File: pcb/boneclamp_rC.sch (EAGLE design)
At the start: 133 parts, among them U1 OPA365AIDBVR, U10 AD5686, U11 LM2663, U12 MAX1735, U13 TLV70245, U14 REF5040MDREP, U15 AD8032ARZ-REEL7, U16 24C, U2 OPA365AIDBVR, U3 OPA365AIDBVR, U4 OPA365AIDBVR, U5 ADS8331IBPW, U6 OPA365AIDBVR, U7 OPA365, U8 OPA365AIDBVR, U9 OPA365AIDBVR

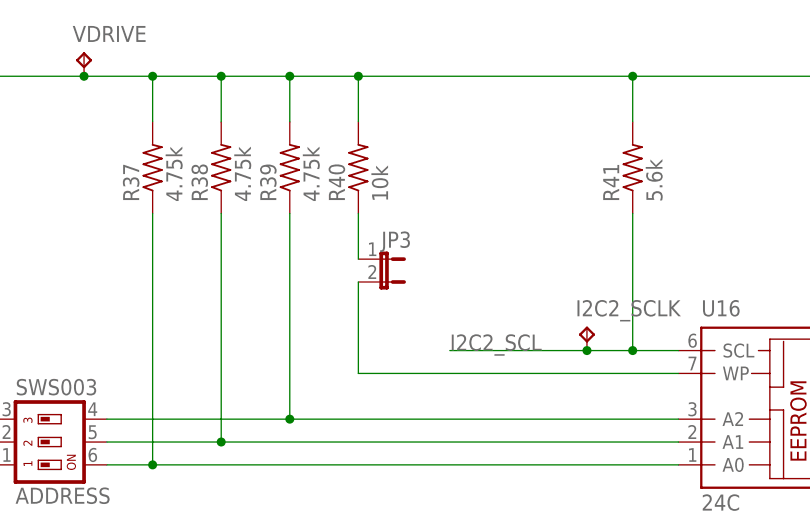
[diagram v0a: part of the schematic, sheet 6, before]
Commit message: Finished basic DAC buffer layout.
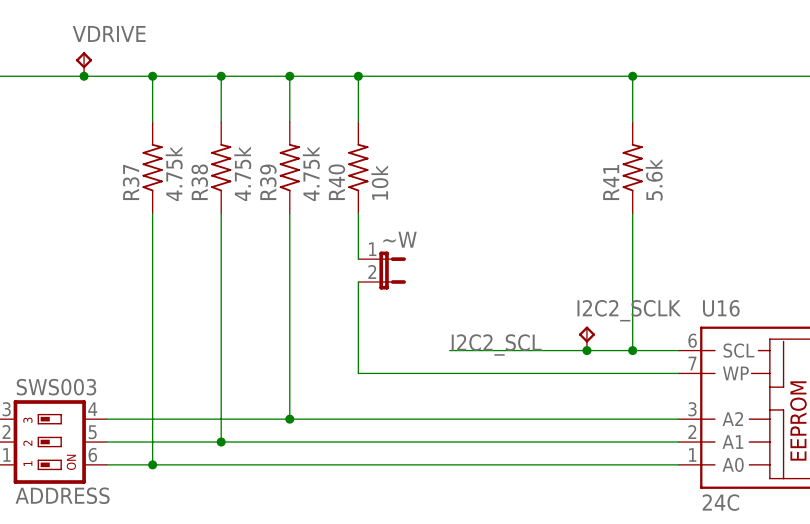
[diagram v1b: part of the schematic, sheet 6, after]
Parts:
- renumbered JP3 to ~W
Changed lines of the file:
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@@
 <part name="SUPPLY10" library="supply2" deviceset="AGND" device=""/>
 <part name="SUPPLY2" library="supply2" deviceset="AGND" device=""/>
-<part name="JP3" library="jumper" deviceset="JP1E" device=""/>
+<part name="~W" library="jumper" deviceset="JP1E" device=""/>
 <part name="ADDRESS" library="smd-special" deviceset="SWS003" device=""/>
 <part name="I2C2_SDA" library="testpad" deviceset="TP" device="B1,27"/>
@@
 <instance part="I2C2_SCLK" gate="G$1" x="-25.4" y="33.02"/>
 <instance part="VDRIVE" gate="G$1" x="-81.28" y="63.5"/>
-<instance part="JP3" gate="A" x="-48.26" y="40.64" rot="R270"/>
+<instance part="~W" gate="A" x="-48.26" y="40.64" rot="R270"/>
 <instance part="ADDRESS" gate="G$1" x="-86.36" y="20.32" rot="MR90"/>
 <instance part="I2C2_SDA" gate="G$1" x="15.24" y="25.4"/>
@@
 <segment>
 <pinref part="R40" gate="G$1" pin="1"/>
-<pinref part="JP3" gate="A" pin="1"/>
+<pinref part="~W" gate="A" pin="1"/>
 <wire x1="-50.8" y1="40.64" x2="-50.8" y2="45.72" width="0.1524" layer="91"/>
 </segment>
@@
 <pinref part="U16" gate="G$1" pin="WP"/>
 <wire x1="-50.8" y1="27.94" x2="-15.24" y2="27.94" width="0.1524" layer="91"/>
-<pinref part="JP3" gate="A" pin="2"/>
+<pinref part="~W" gate="A" pin="2"/>
 <wire x1="-50.8" y1="27.94" x2="-50.8" y2="38.1" width="0.1524" layer="91"/>
 </segment>
